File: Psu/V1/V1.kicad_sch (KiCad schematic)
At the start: 0 parts

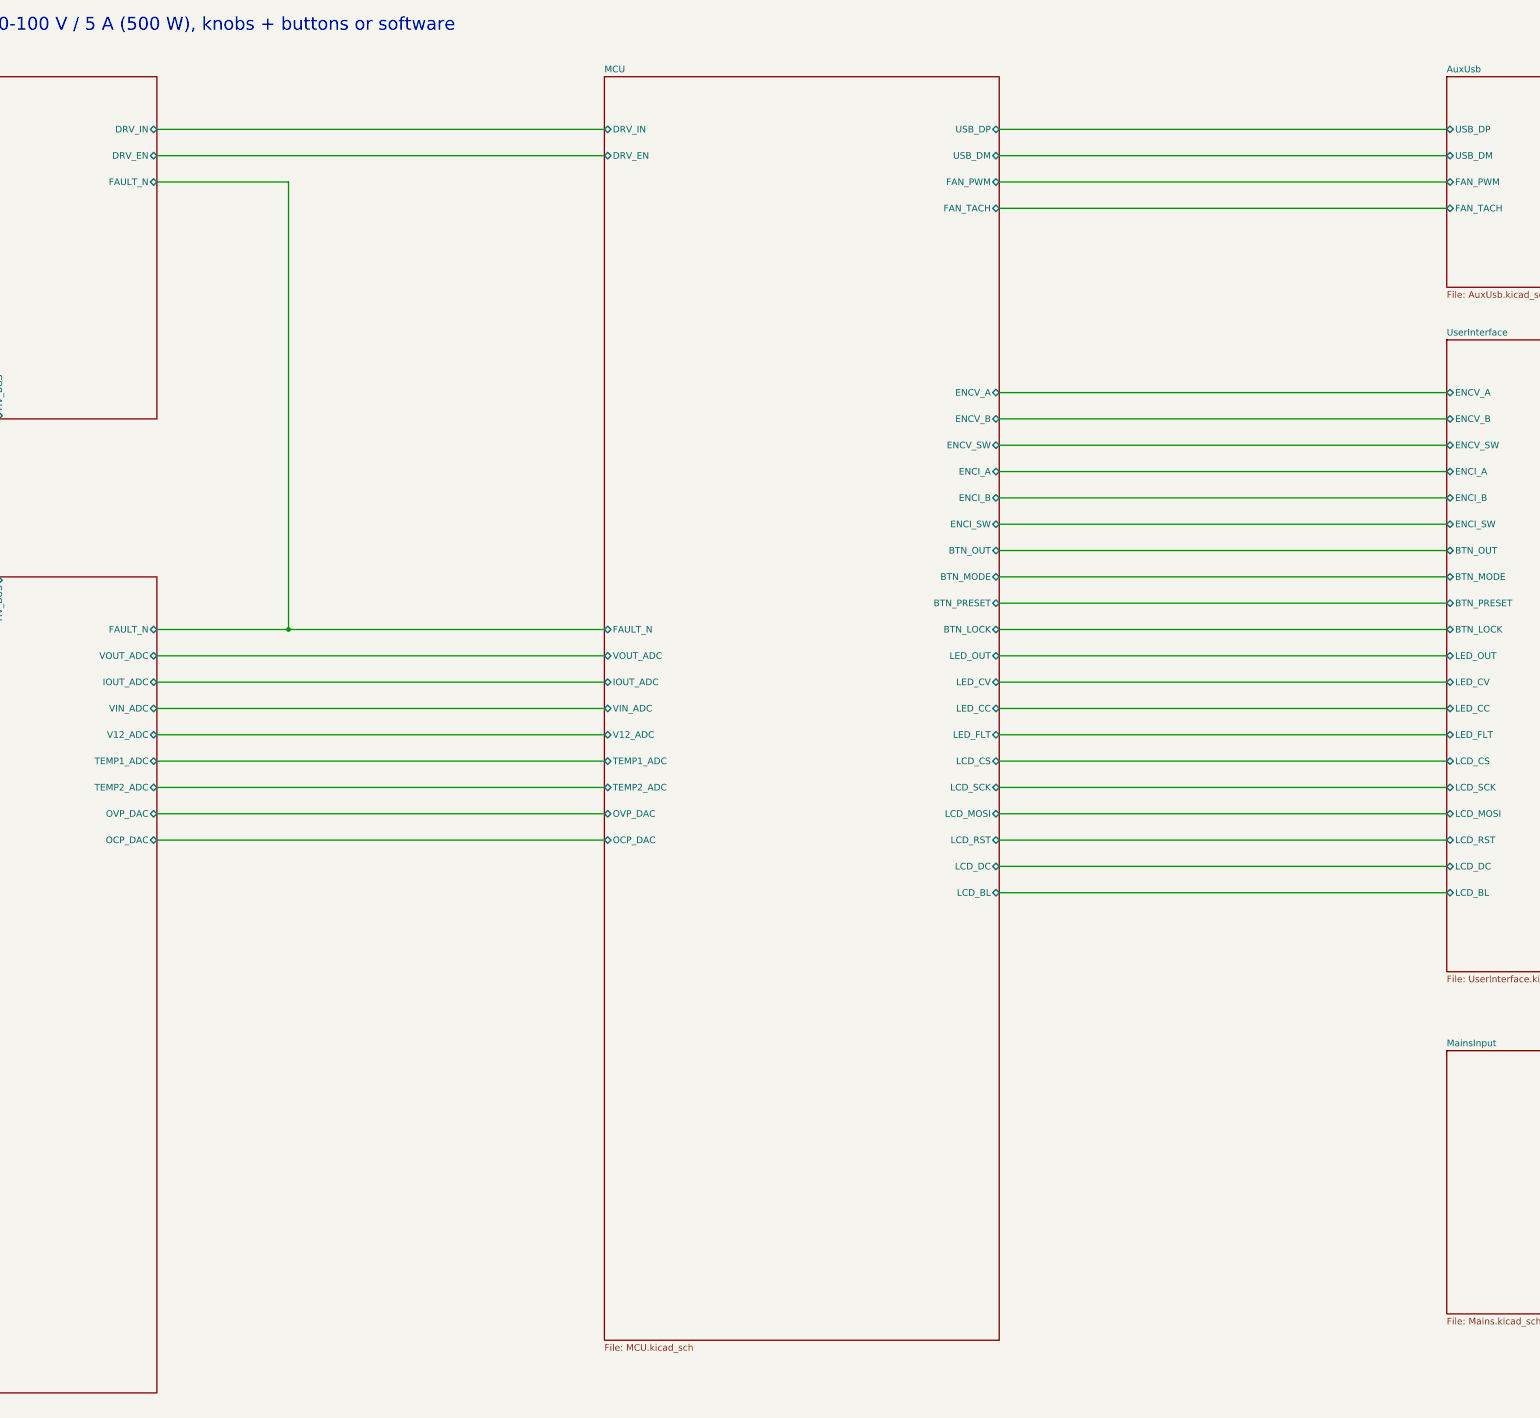
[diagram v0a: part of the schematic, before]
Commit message: Jfjja
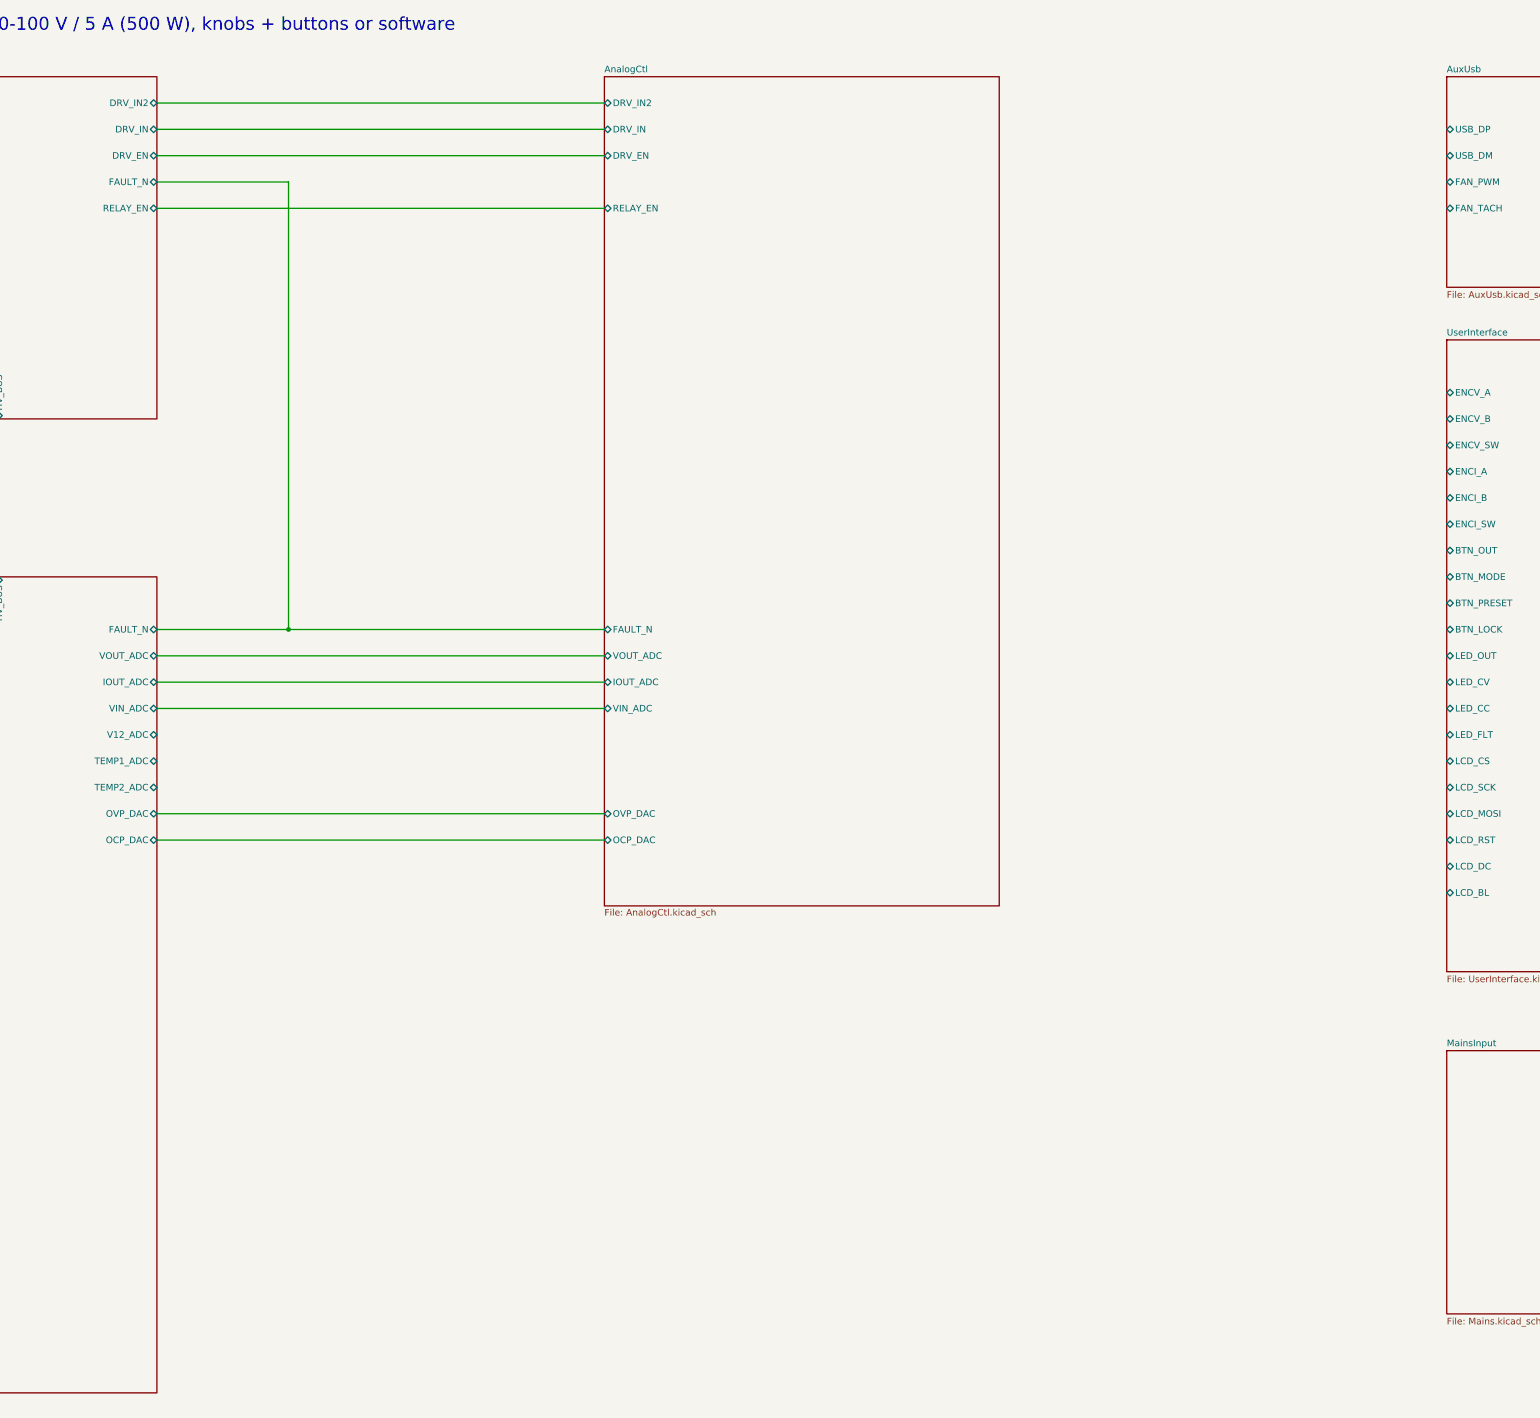
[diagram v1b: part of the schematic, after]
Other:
- sheet MCU renamed AnalogCtl
- sheet AnalogCtl: file MCU.kicad_sch -> AnalogCtl.kicad_sch
- sheet AnalogCtl ports: added DRV_IN2, RELAY_EN; removed BTN_LOCK, BTN_MODE, BTN_OUT, BTN_PRESET, ENCI_A, ENCI_B, ENCI_SW, ENCV_A, ENCV_B, ENCV_SW, FAN_PWM, FAN_TACH, LCD_BL, LCD_CS, LCD_DC, LCD_MOSI, LCD_RST, LCD_SCK, LED_CC, LED_CV, LED_FLT, LED_OUT, TEMP1_ADC, TEMP2_ADC, USB_DM, USB_DP, V12_ADC
- sheet PowerStage ports: added DRV_IN2, RELAY_EN; removed none
